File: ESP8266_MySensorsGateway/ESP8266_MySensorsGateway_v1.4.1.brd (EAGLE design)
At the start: 50 x 24.9 mm, 39 parts, among them IC1 3V3, IC4 ATSHA204A

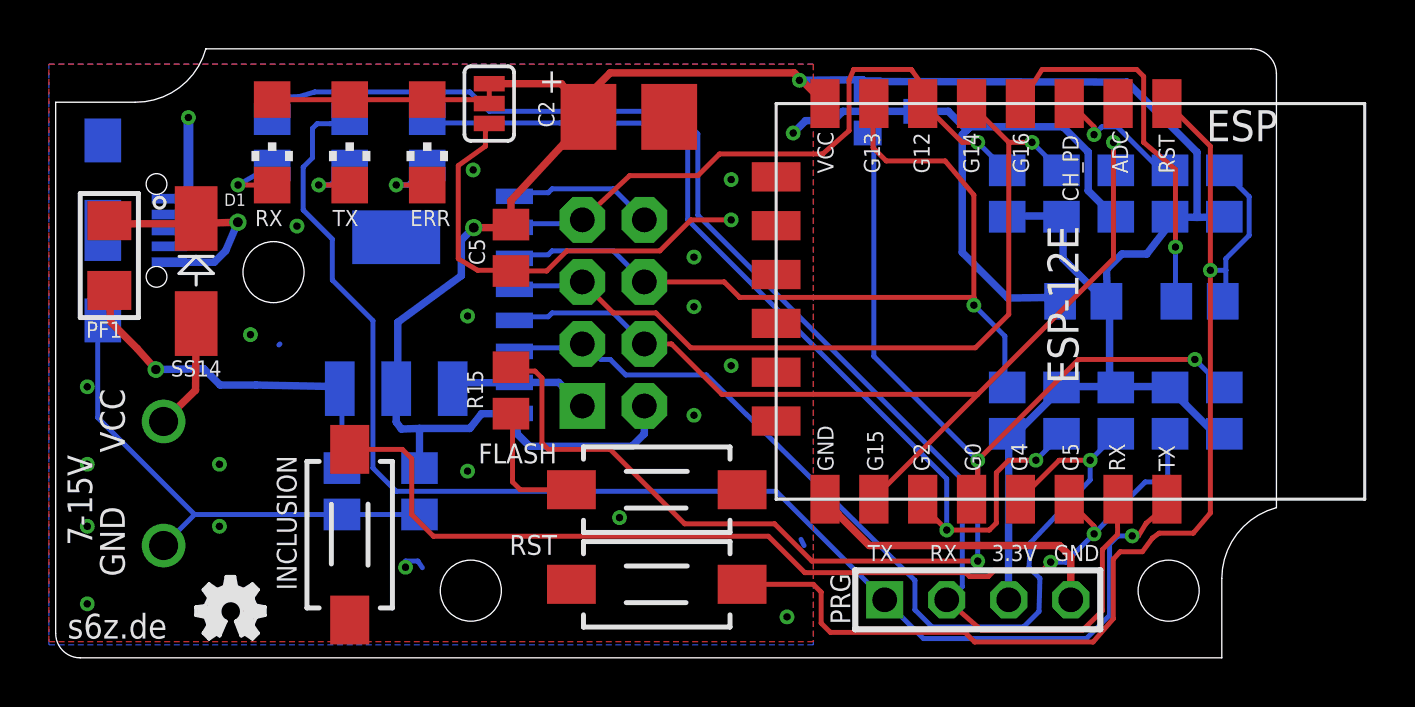
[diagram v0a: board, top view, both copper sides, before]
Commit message: .
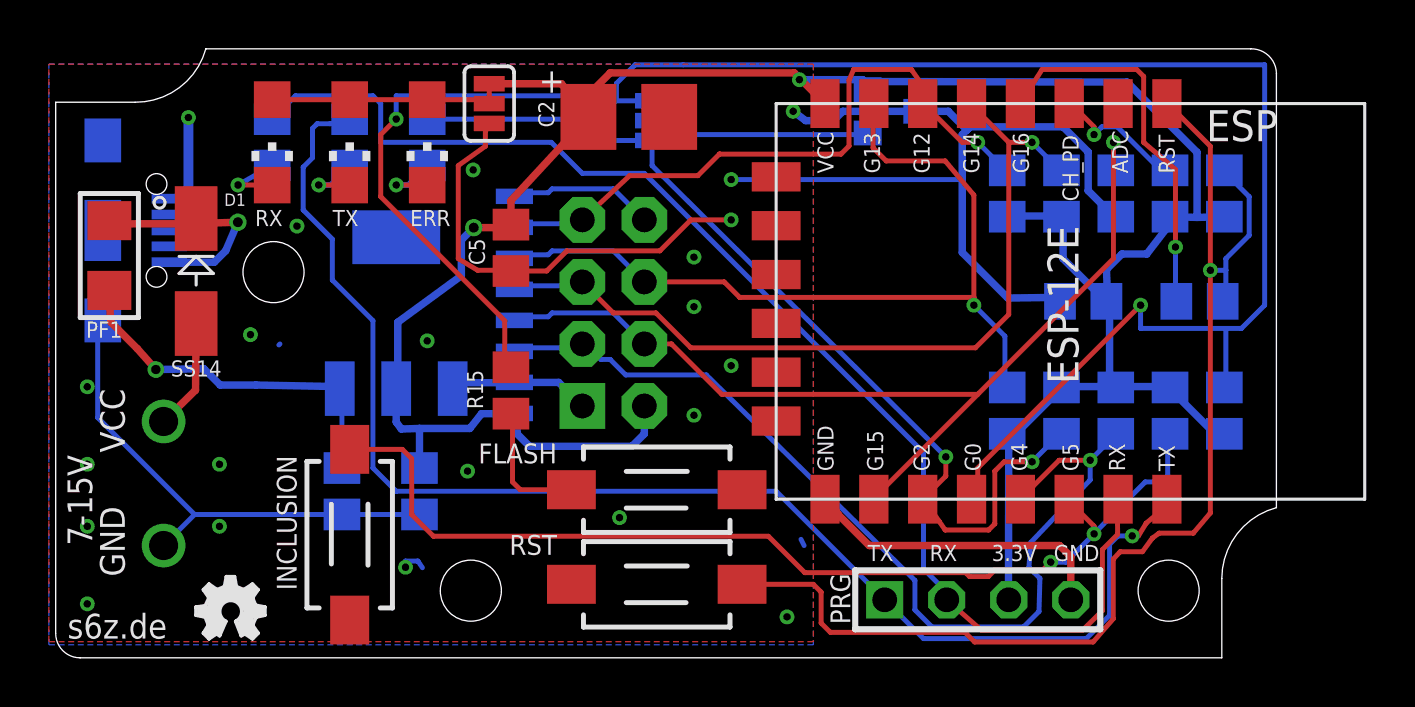
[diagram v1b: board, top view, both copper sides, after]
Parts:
- added SJ2, SJ3: JUMPER-PAD-3-NOYES_SILK, SparkFun-Passives:PAD-JUMPER-3-NO_YES_SILK
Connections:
- new net D3: ESP.12, R15.2, R5.1, SJ2.3, SJ3.1
- new net D4: ESP.11, R4.1, SJ2.1, SJ3.3
- net ATSHA: now also SJ2.2; no longer ESP.12, R15.2, R5.1
- net LED_ERR: now also SJ3.2; no longer ESP.11, R4.1
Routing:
- net D3: track 0.00 -> 81.6 mm, vias 0 -> 2
- net ATSHA: track 57.4 -> 9.49 mm, vias 3 -> 0
- net LED_ERR: track 40.8 -> 6.38 mm, vias 2 -> 0
- net D4: track 0.00 -> 32.1 mm, vias 0 -> 2
- net GND: track 91.7 -> 101.1 mm
- net RXD: track 54.8 -> 52.5 mm
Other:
- board text added: "ATSHA"
- board text added: "D3/G0"
- board text added: "D4/G2"
- board text added: "LED"
